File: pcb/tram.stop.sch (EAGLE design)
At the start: 22 parts, among them Q1 BC847SMD, U1 ATTINY85V-10SU, U2 LM1117MP-5.0

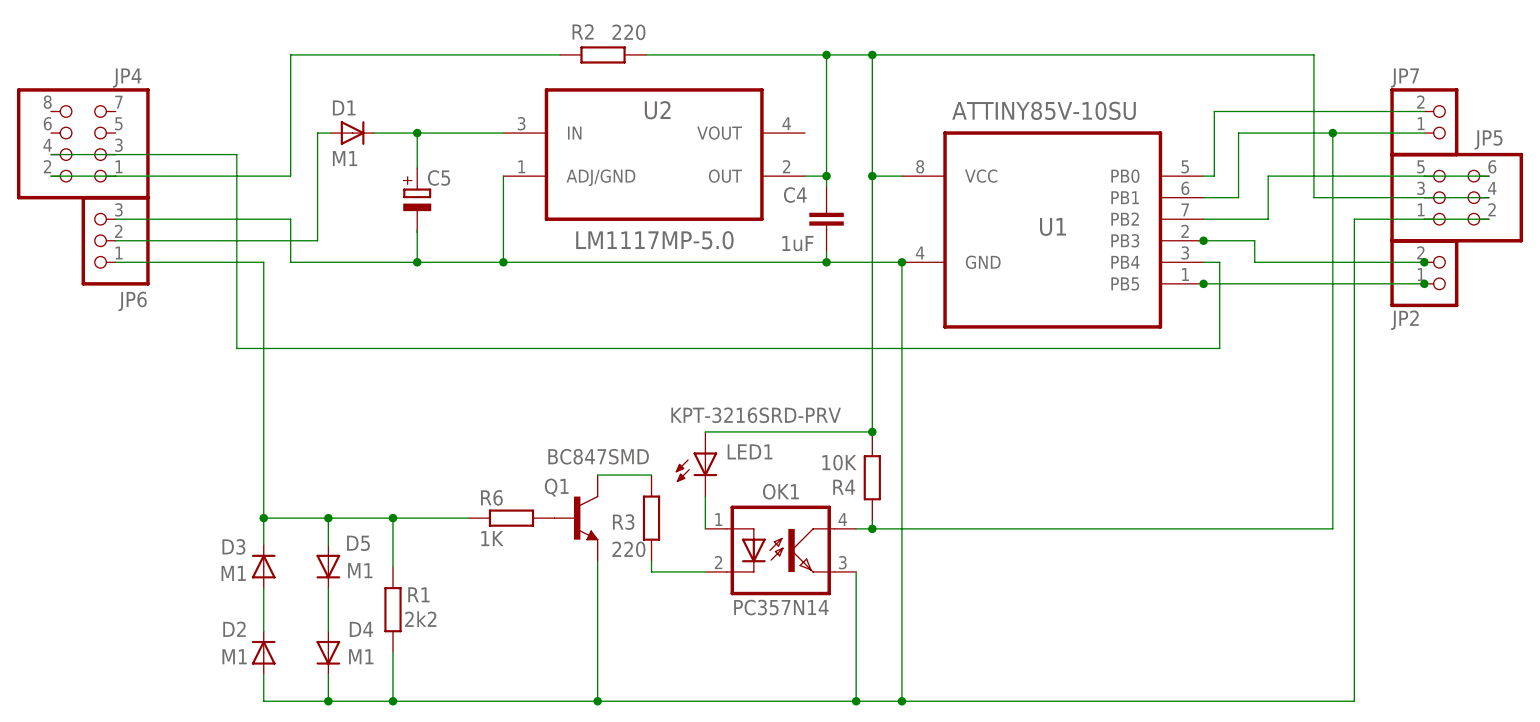
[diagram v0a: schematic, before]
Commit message: #! finalize code
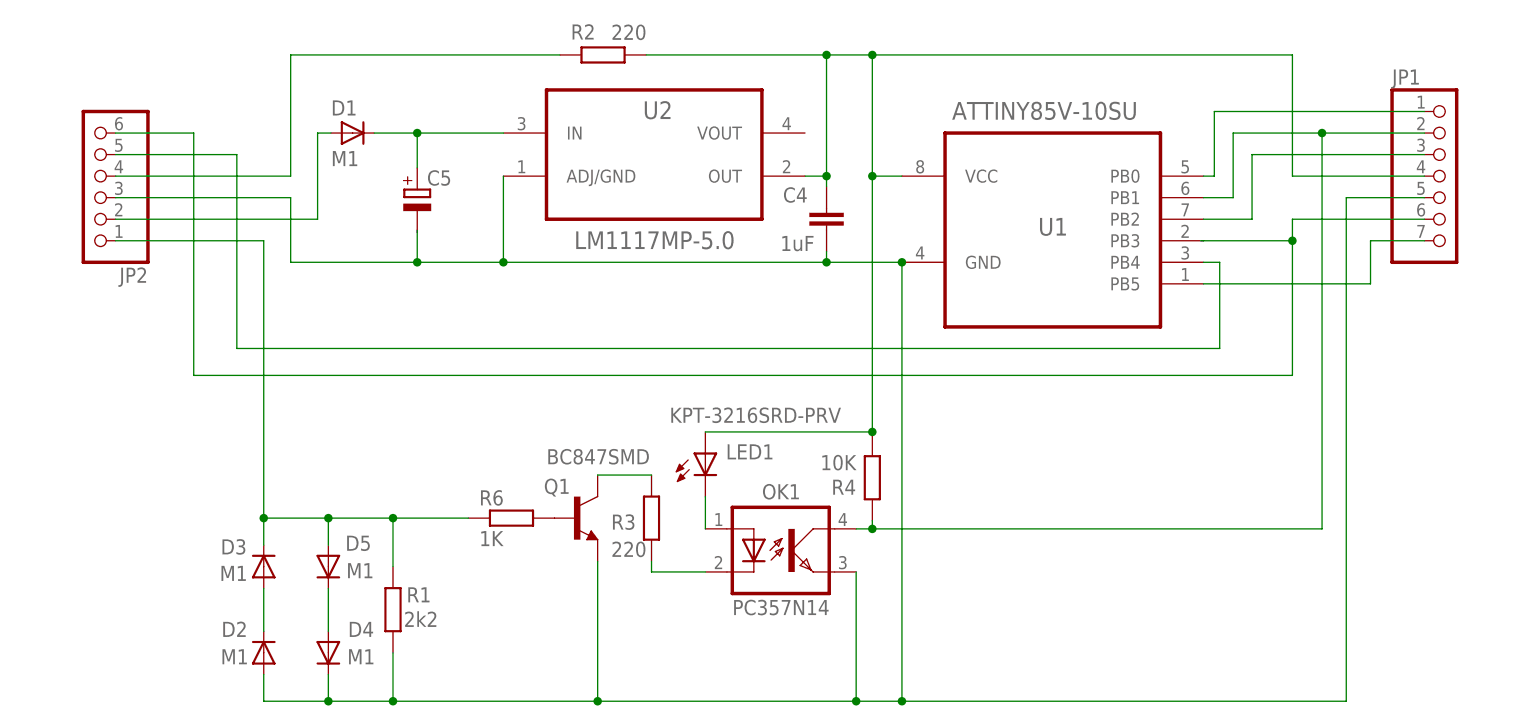
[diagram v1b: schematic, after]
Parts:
- removed JP4: (no value), pinhead:PINHD-2X4/90
- removed JP5: (no value), pinhead:PINHD-2X3/90
- removed JP6: (no value), pinhead:PINHD-1X3/90
- removed JP7: (no value), pinhead:PINHD-1X2/90
- added JP1: (no value), pinhead:PINHD-1X7
- JP2: device pinhead:PINHD-1X2/90 -> pinhead:PINHD-1X6/90
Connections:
- removed net N$1: JP2.1, U1.PB5
- new net N$13: JP1.6, JP2.6
- new net N$16: JP1.7, U1.PB5
- net JP1: now also JP2.1; no longer JP6.1
- net JP2: now also JP1.5, JP2.3; no longer JP5.1, JP5.2, JP6.3
- net N$10: now also JP1.3; no longer JP5.5, JP5.6
- net N$11: now also JP1.1; no longer JP7.2
- net N$12: now also JP2.4; no longer JP4.1, JP4.2
- net N$14: now also JP1.2; no longer JP7.1
- net N$15: now also JP1.4; no longer JP5.3, JP5.4
- net N$2: no longer JP2.2
- net N$21: now also JP2.2; no longer JP6.2
- net RED2: now also JP2.5; no longer JP4.3, JP4.4
